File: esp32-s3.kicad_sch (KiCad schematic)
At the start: 9 parts, among them SW1 BOOT, SW2 RESET, U1 ESP32-S3-WROOM-1

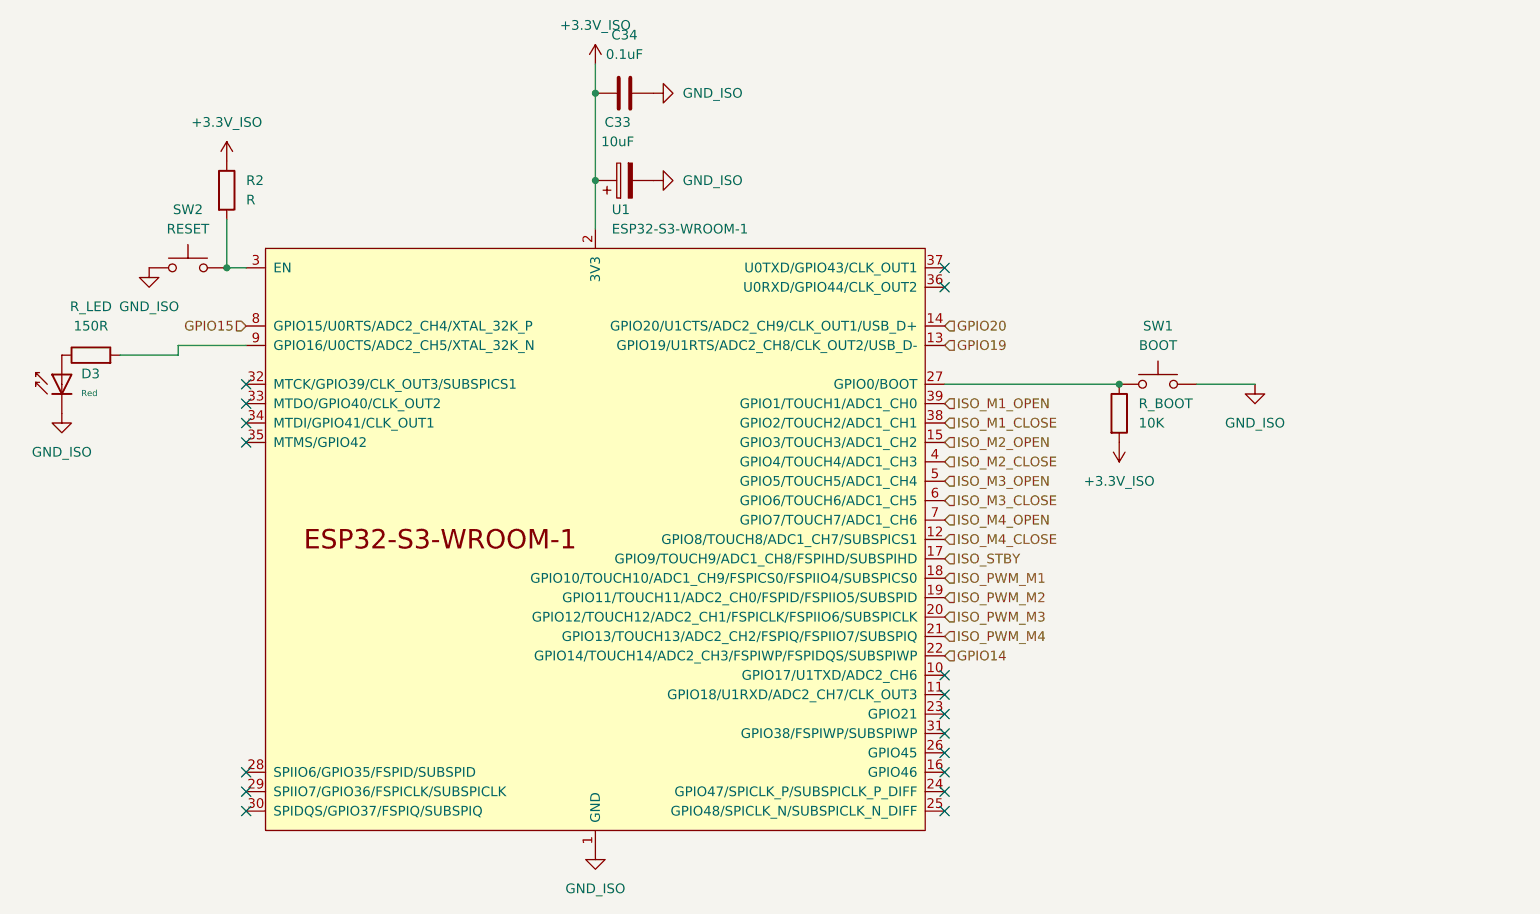
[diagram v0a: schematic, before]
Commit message: Started running traces
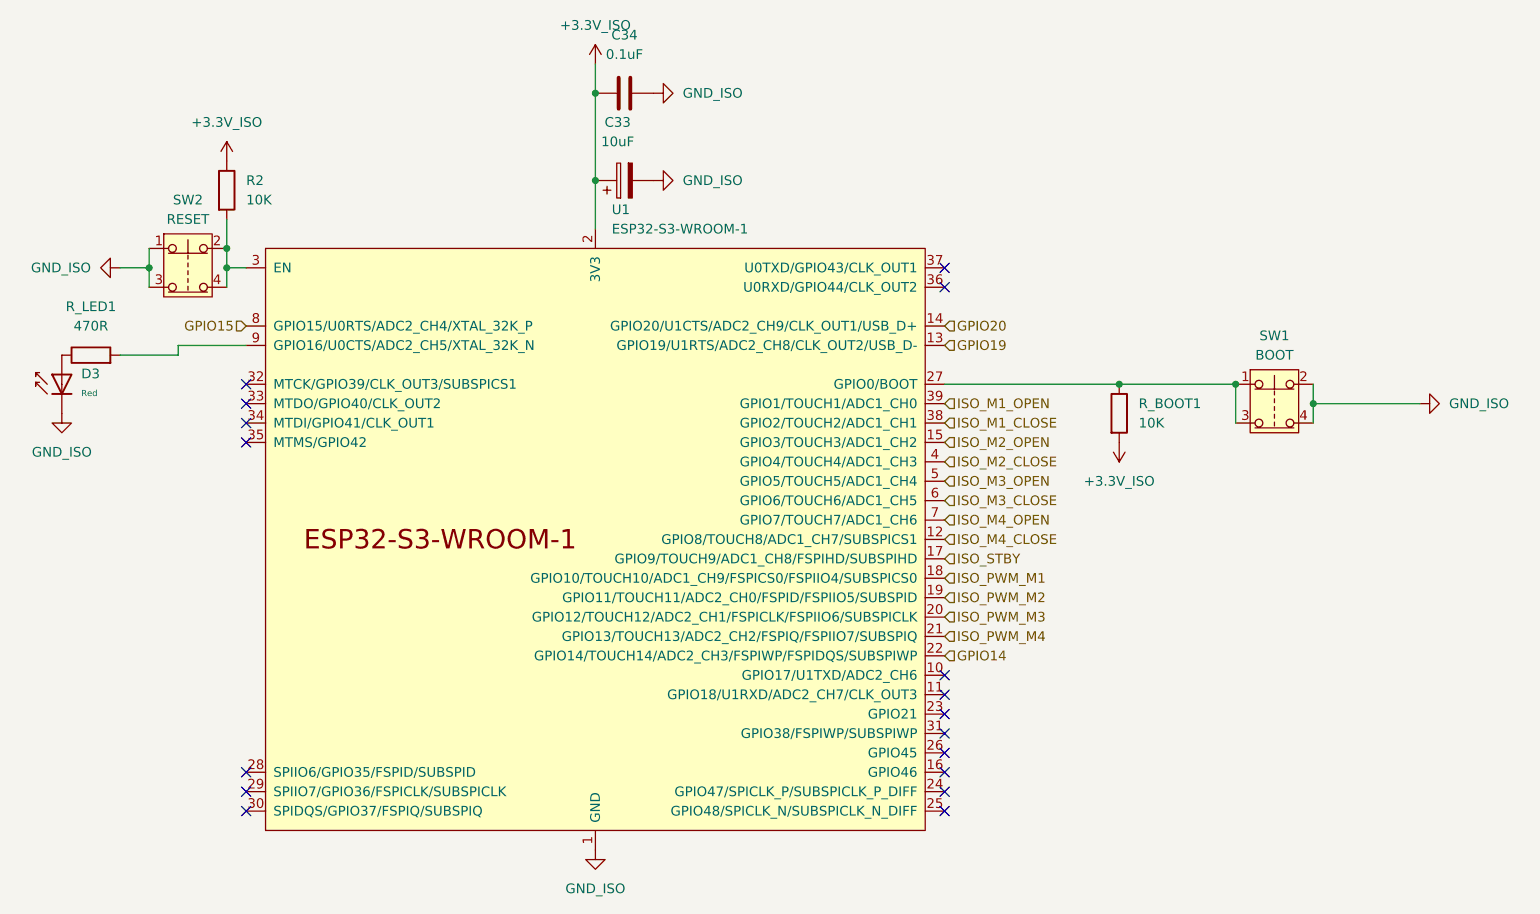
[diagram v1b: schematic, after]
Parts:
- C33: footprint (none) -> Capacitor_SMD:C_0805_2012Metric
- C34: footprint (none) -> Capacitor_SMD:C_0603_1608Metric
- R2: value R -> 10K; footprint (none) -> Resistor_SMD:R_0603_1608Metric
- R_BOOT1: renamed from R_BOOT; footprint (none) -> Resistor_SMD:R_0603_1608Metric
- R_LED1: renamed from R_LED; value 150R -> 470R; footprint (none) -> Resistor_SMD:R_0603_1608Metric
- SW1, SW2: footprint (none) -> barn_shade_controller:SW-SMD_4P-L3.5-W3.0-P1.50-LS4.7; symbol Switch:SW_Push -> Switch:SW_Push_Open_Dual
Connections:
- net GND_ISO: now also SW1.4, SW2.3
- net at R2.2, SW2.2, U1.3 (EN): now also SW2.4
- net at R_BOOT1.1, SW1.1, U1.27 (GPIO0/BOOT): now also SW1.3
